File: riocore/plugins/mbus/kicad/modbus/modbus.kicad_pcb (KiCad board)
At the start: 2 copper layers, 12 x 19.5 mm, 6 parts, among them U12 MAX485E

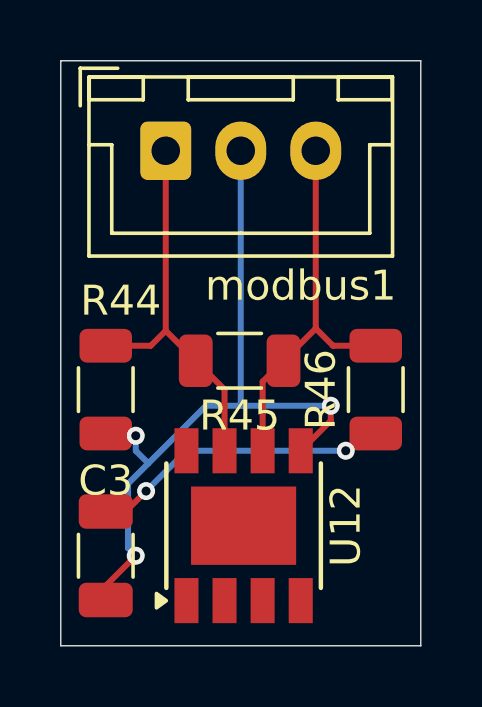
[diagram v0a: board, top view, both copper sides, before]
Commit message: kicad: module selection / some fixes
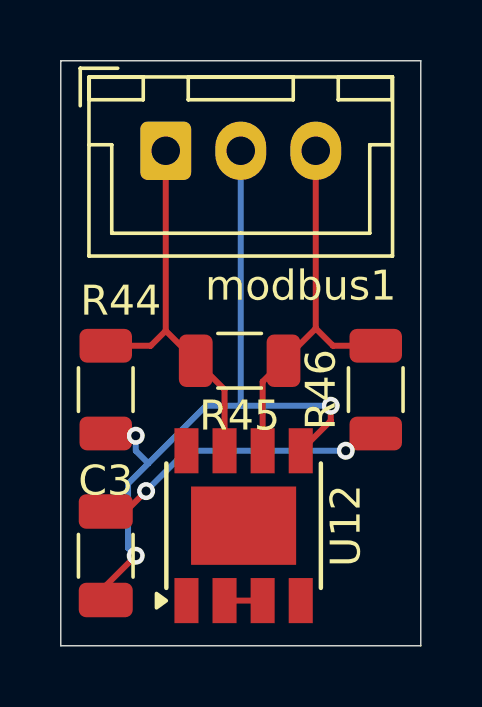
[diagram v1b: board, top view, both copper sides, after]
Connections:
- net /rw renamed /tx_enable
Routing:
- net /tx_enable: track 0.00 -> 1.27 mm
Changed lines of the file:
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@@
 	(net 4 "Net-(U12-B)")
 	(net 5 "/rx")
-	(net 6 "/rw")
+	(net 6 "/tx_enable")
 	(net 7 "/tx")
 	(footprint "Package_SO:Diodes_SO-8EP"
@@
 			(size 1.505 0.802)
 			(layers "F.Cu" "F.Mask" "F.Paste")
-			(net 6 "/rw")
+			(net 6 "/tx_enable")
 			(pinfunction "~{RE}")
 			(pintype "input")
@@
 			(size 1.505 0.802)
 			(layers "F.Cu" "F.Mask" "F.Paste")
-			(net 6 "/rw")
+			(net 6 "/tx_enable")
 			(pinfunction "DE")
 			(pintype "input")
@@
 		(net 4)
 	)
+	(segment
+		(start 145.96 95.495)
+		(end 147.23 95.495)
+		(width 0.2)
+		(layer "F.Cu")
+		(net 6)
+	)
 	(embedded_fonts no)
